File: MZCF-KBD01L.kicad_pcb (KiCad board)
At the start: 2 copper layers, 142.1 x 127.8 mm, 78 parts, among them CN1 XH-4AW_C2908613, SW1 SW_Push, SW10 SW_Push, SW11 SW_Push, SW12 SW_Push, SW13 SW_Push, SW15 SW_Push, SW16 SW_Push, SW17 SW_Push, SW18 SW_Push, SW19 SW_Push, SW2 SW_Push, SW20 SW_Push, SW22 SW_Push, SW23 SW_Push, SW24 SW_Push, SW25 SW_Push, SW26 SW_Push, SW27 SW_Push, SW29 SW_Push, SW3 SW_Push, SW30 SW_Push, SW31 SW_Push, SW32 SW_Push, SW33 SW_Push, SW37 SW_Push, SW38 SW_Push, SW39 SW_Push, SW4 SW_Push, SW40 SW_Push, SW5 SW_Push, SW6 SW_Push, SW8 SW_Push, SW9 SW_Push, U1 RP2040-ZERO

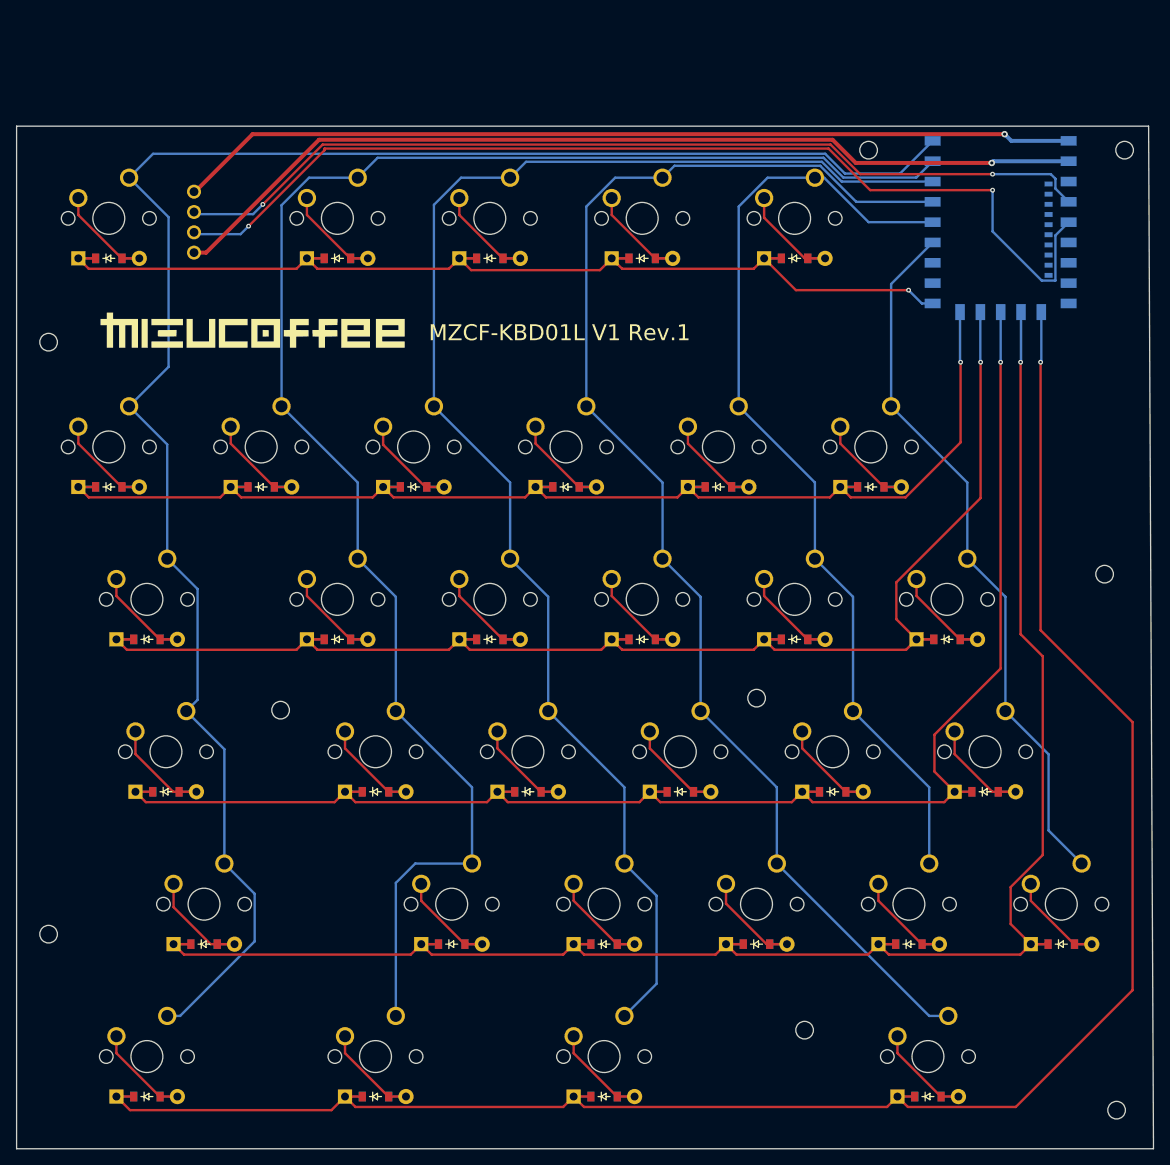
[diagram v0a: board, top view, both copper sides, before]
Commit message: feat: new left keyboard
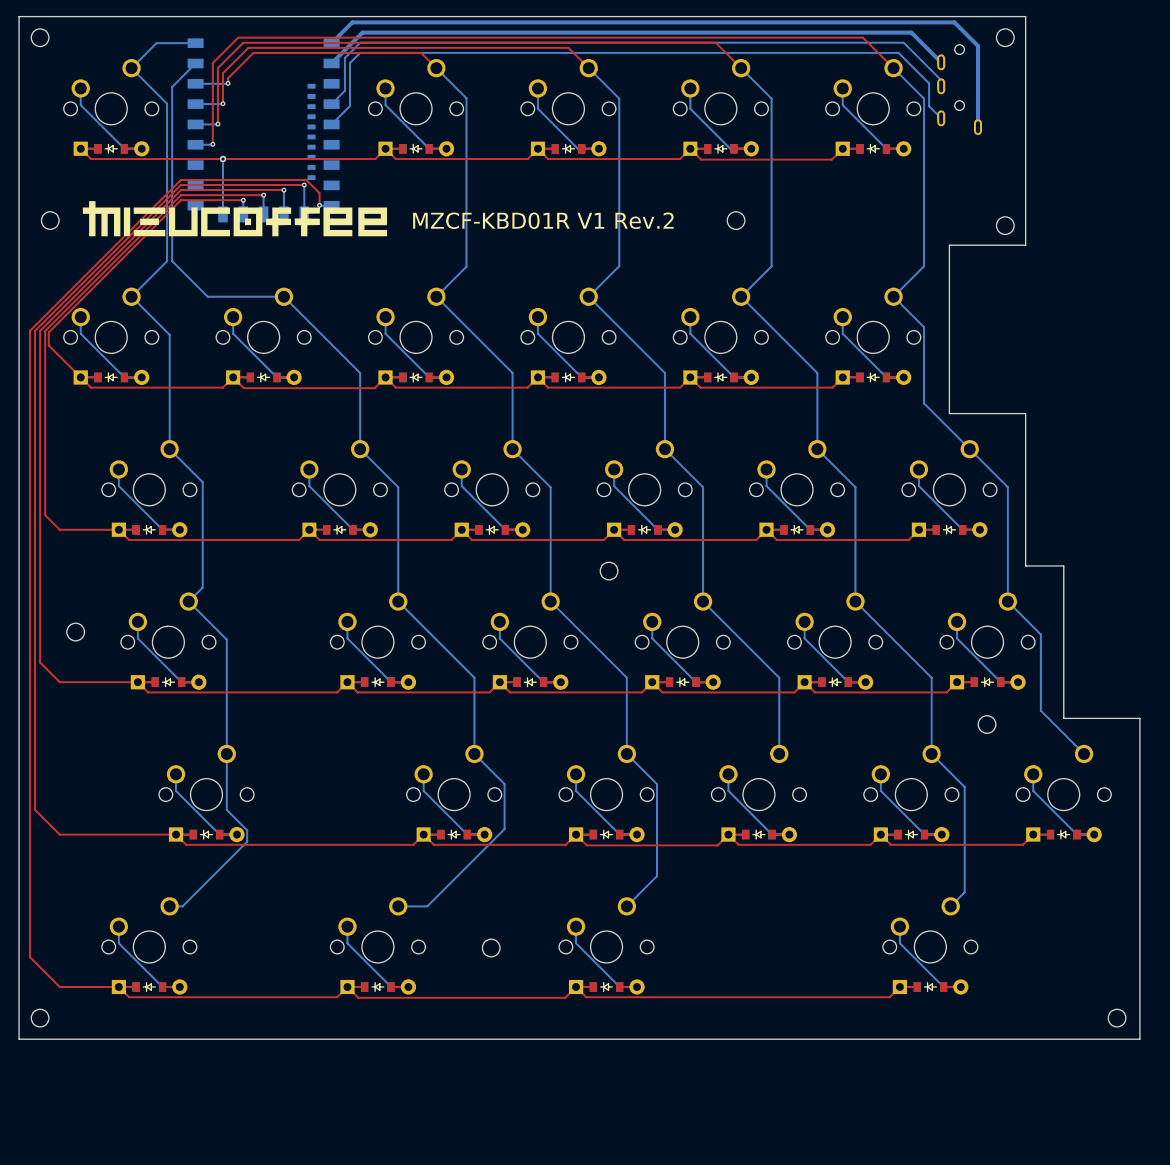
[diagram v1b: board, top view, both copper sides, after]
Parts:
- removed D24, D37, D38, D39, D40: 1N4148W, ComboDiode
- removed SW24, SW37, SW38, SW39, SW40: SW_Push, MX
- added D14: 1N4148W, ComboDiode, B.Cu at (74.9, 70.4)
- added D21: 1N4148W, ComboDiode, B.Cu at (103.5, 89.5)
- added D28: 1N4148W, ComboDiode, B.Cu at (127.3, 108.5)
- added D34: 1N4148W, ComboDiode, B.Cu at (146.4, 108.5)
- added D35: 1N4148W, ComboDiode, B.Cu at (155.9, 127.6)
- added H10: MountingHole_2.2mm_M2, MountingHole:MountingHole_2.2mm_M2, F.Cu at (27.9, 150.5)
- added H11: MountingHole_2.2mm_M2, MountingHole:MountingHole_2.2mm_M2, F.Cu at (162.6, 150.5)
- added SW14: SW_Push, MX, F.Cu at (74.9, 65.4)
- added SW21: SW_Push, MX, F.Cu at (103.5, 84.5)
- added SW28: SW_Push, MX, F.Cu at (127.3, 103.5)
- added SW34: SW_Push, MX, F.Cu at (146.4, 103.5)
- added SW35: SW_Push, MX, F.Cu at (155.9, 122.6)
- CN1: value XH-4AW_C2908613 -> PJ-320A_C49284721; footprint lcsc_footprints:C2908613_CONN-TH_XH-4AW -> lcsc_footprints:C49284721_AUDIO-TH_PJ-320A_C49284721
- moved D13 118.6 mm to (74.9, 41.8), turned to 0 degrees
- moved SW13 118.6 mm to (74.9, 36.8)
- moved H5 109.0 mm to (148.6, 51.4)
- moved H1 104.5 mm to (27.9, 27.9)
- moved D19 99.5 mm to (94.0, 41.8), turned to 0 degrees
- moved SW19 99.5 mm to (94.0, 36.8)
- moved CN1 97.0 mm to (142.9, 35.1)
- moved U1 92.9 mm to (55.9, 39.3)
- moved D20 90.0 mm to (94.0, 70.4), turned to 0 degrees
- moved SW20 90.0 mm to (94.0, 65.4)
- moved H9 80.8 mm to (84.3, 141.7)
- moved D25 80.5 mm to (113.0, 41.8), turned to 0 degrees
- moved SW25 80.5 mm to (113.0, 36.8)
- moved D29 73.5 mm to (136.8, 127.6), turned to 0 degrees
- moved SW29 73.5 mm to (136.8, 122.6)
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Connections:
- CN1 pad 2: Net-(U1-GP29) -> Net-(U1-5V)
- CN1 pad 3: Net-(U1-GP28) -> Net-(U1-GP29)
- CN1 pad 4: Net-(U1-GND) -> Net-(U1-GP28)
- D10 pad 1: /ROW2 -> /ROW3
- D11 pad 1: /ROW3 -> /ROW4
- D12 pad 1: /ROW4 -> /ROW5
- D13 pad 1: /ROW5 -> /ROW0
- D15 pad 1: /ROW0 -> /ROW2
- D16 pad 1: /ROW1 -> /ROW3
- D17 pad 1: /ROW2 -> /ROW4
- D18 pad 1: /ROW3 -> /ROW5
- D19 pad 1: /ROW4 -> /ROW0
- D20 pad 1: /ROW5 -> /ROW1
- D22 pad 1: /ROW0 -> /ROW3
- D23 pad 1: /ROW1 -> /ROW4
- D25 pad 1: /ROW3 -> /ROW0
- D26 pad 1: /ROW4 -> /ROW1
- D27 pad 1: /ROW5 -> /ROW2
- D29 pad 1: /ROW0 -> /ROW4
- D30 pad 1: /ROW1 -> /ROW5
- D31 pad 1: /ROW2 -> /ROW0
- D32 pad 1: /ROW3 -> /ROW1
- D33 pad 1: /ROW4 -> /ROW2
- D8 pad 1: /ROW0 -> /ROW1
- D9 pad 1: /ROW1 -> /ROW2
- SW13 pad 1: /COL1 -> /COL2
- SW19 pad 1: /COL2 -> /COL3
- SW20 pad 1: /COL2 -> /COL3
- SW25 pad 1: /COL3 -> /COL4
- SW26 pad 1: /COL3 -> /COL4
- SW27 pad 1: /COL3 -> /COL4
- SW31 pad 1: /COL4 -> /COL5
- SW32 pad 1: /COL4 -> /COL5
- SW33 pad 1: /COL4 -> /COL5
- U1 pad 10: /ROW1 -> /ROW0
- U1 pad 11: /ROW2 -> /ROW1
- U1 pad 12: /ROW3 -> /ROW2
- U1 pad 13: /ROW4 -> /ROW3
- U1 pad 14: /ROW5 -> /ROW4
- U1 pad 15: /ROW6 -> /ROW5
- U1 pad 17: unconnected-(U1-GP26-Pad17) -> Net-(U1-GP26)
- U1 pad 18: unconnected-(U1-GP27-Pad18) -> Net-(U1-GP27)
- U1 pad 9: /ROW0 -> /BTN1
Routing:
- net /COL5: track 89.6 -> 199.1 mm, vias 0 -> 1
- net /COL0: track 226.6 -> 130.2 mm
- net /COL4: track 120.0 -> 198.1 mm, vias 0 -> 1
- net /COL1: track 205.0 -> 137.0 mm
- net Net-(U1-GP28): track 130.2 -> 88.1 mm, vias 2 -> 0
- net /ROW4: track 221.4 -> 262.1 mm
- net Net-(U1-GND): track 116.5 -> 79.3 mm, vias 1 -> 0
- net Net-(U1-GP29): track 116.7 -> 85.0 mm, vias 2 -> 0
- net /ROW3: track 198.1 -> 229.1 mm
- net /COL2: track 180.2 -> 153.7 mm, vias 0 -> 1
- net /ROW2: track 177.7 -> 201.0 mm
- net Net-(U1-5V): track 112.7 -> 93.6 mm, vias 1 -> 0
- net Net-(D34-A): track 0.00 -> 16.3 mm
- net Net-(D28-A): track 0.00 -> 16.3 mm
- net Net-(D21-A): track 0.00 -> 16.3 mm
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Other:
- board size 142.1 x 127.8 mm -> 140.1 x 127.8 mm
- board text added: "MZCF-KBD01R V1 Rev.2"
- board text removed: "MZCF-KBD01L V1 Rev.1"
